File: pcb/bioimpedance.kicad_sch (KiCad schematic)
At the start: 44 parts, among them J1 Conn_01x05_Pin, J3 USB_C_Receptacle_USB2.0_16P, J6 Conn_01x16_Pin, J8 Conn_01x16_Pin, SW5 SW_Push, SW6 SW_Push, U1 ESP32-S3-WROOM-1, U2 MAX30001CWV_T, U3 AP2112K-3.3, U4 AP2112K-1.8, Y1 OK322532.768KJBA4SL

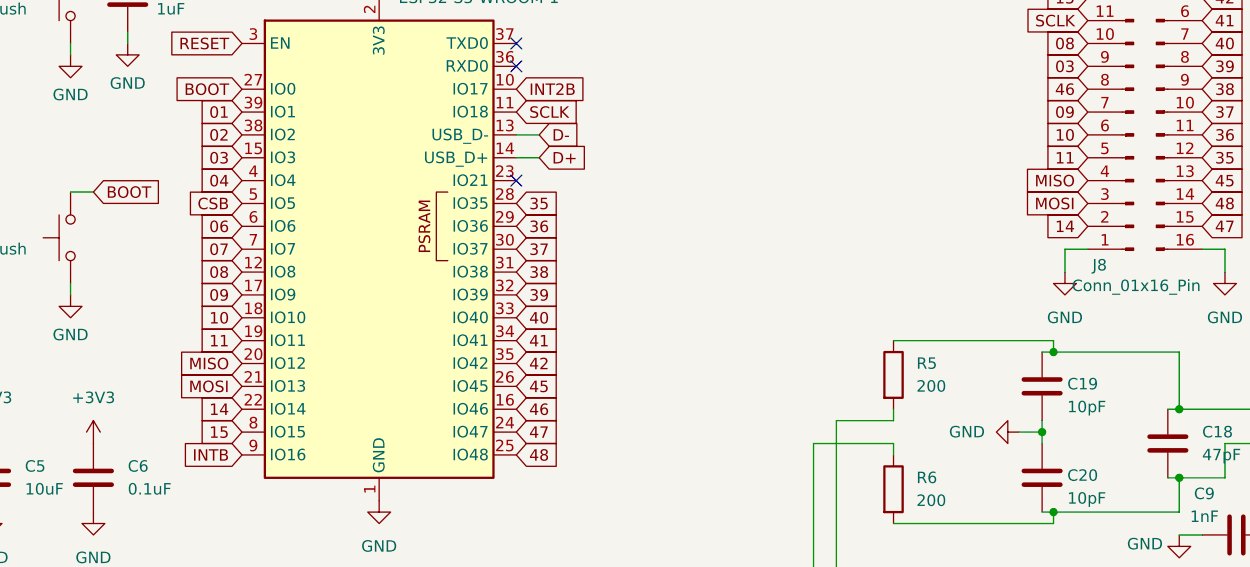
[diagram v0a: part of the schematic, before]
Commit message: reroute pcb AGAIN
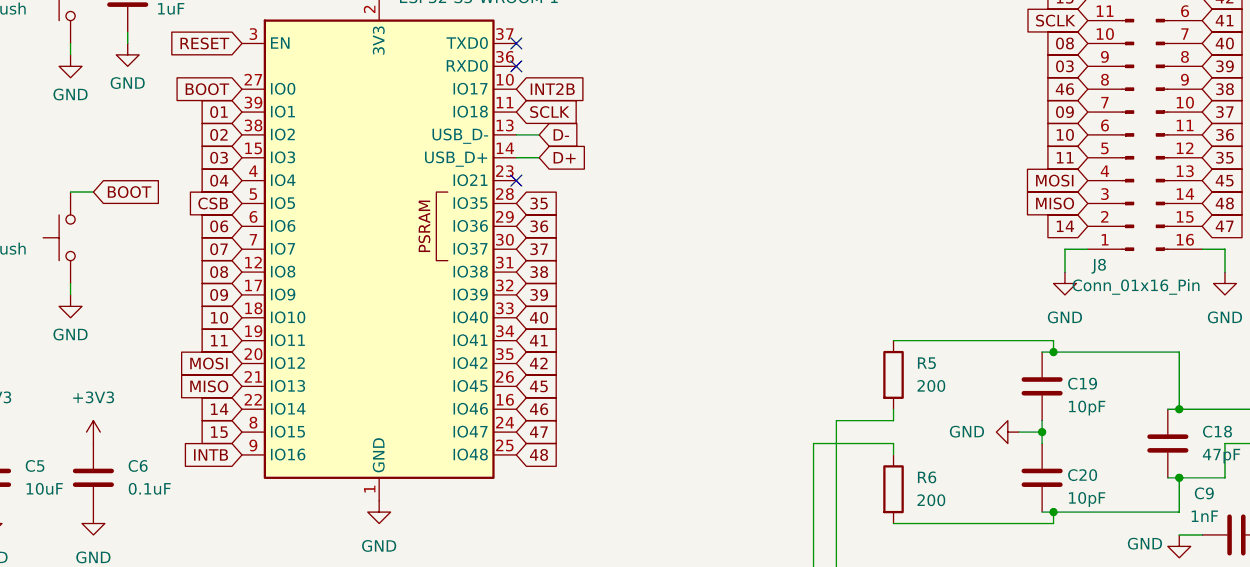
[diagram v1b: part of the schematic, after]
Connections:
- net MISO: now also J8.3 (Pin_3), U1.21 (IO13); no longer J8.4 (Pin_4), U1.20 (IO12)
- net MOSI: now also J8.4 (Pin_4), U1.20 (IO12); no longer J8.3 (Pin_3), U1.21 (IO13)

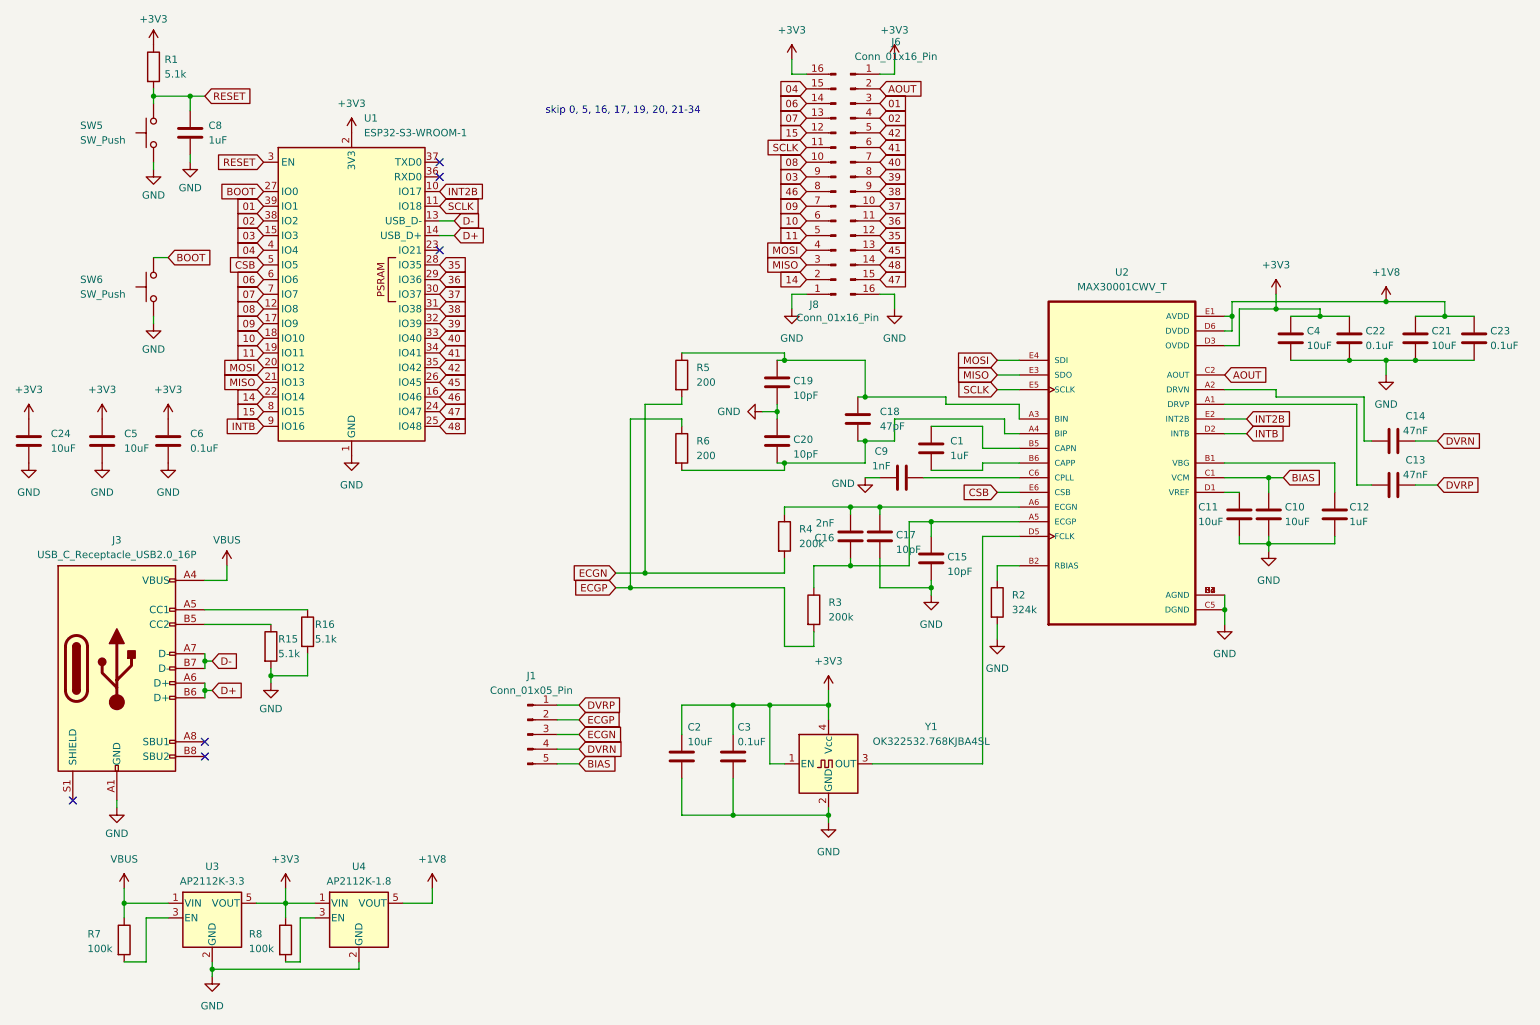
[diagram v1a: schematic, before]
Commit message: reroute board. again
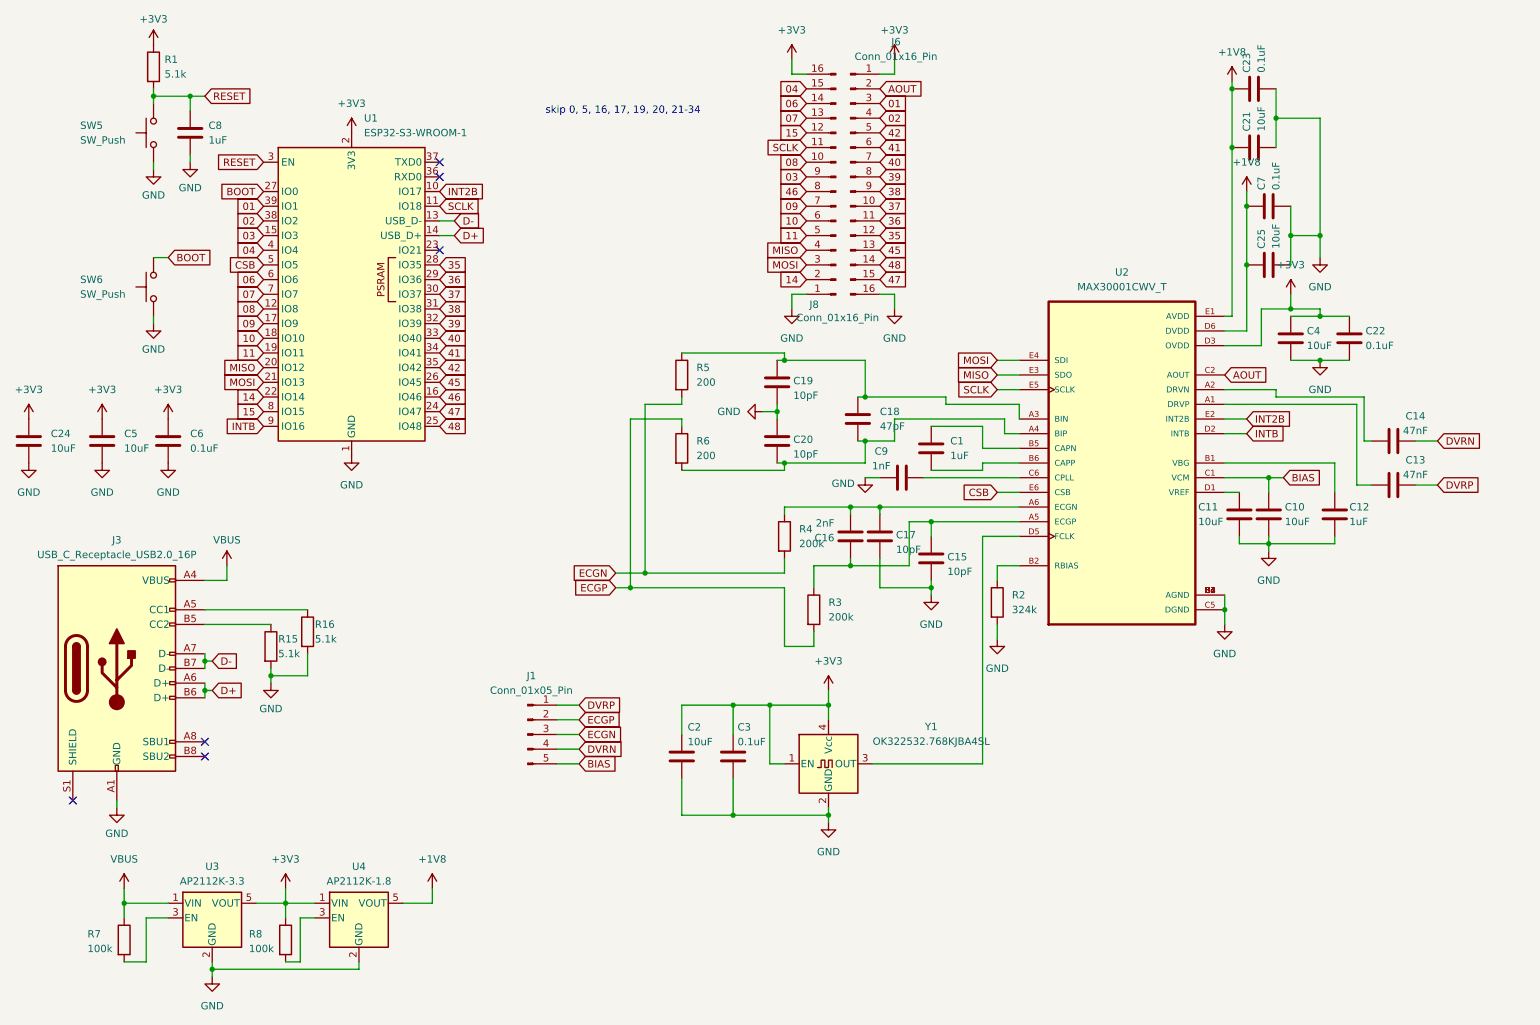
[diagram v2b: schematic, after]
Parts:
- added C25: 10uF, Capacitor_SMD:C_0805_2012Metric, symbol Device:C
- added C7: 0.1uF, Capacitor_SMD:C_0805_2012Metric, symbol Device:C
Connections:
- net +1V8: now also C25.1, C7.1
- net GND: now also C25.2, C7.2
- net MISO: now also J8.4 (Pin_4), U1.20 (IO12); no longer J8.3 (Pin_3), U1.21 (IO13)
- net MOSI: now also J8.3 (Pin_3), U1.21 (IO13); no longer J8.4 (Pin_4), U1.20 (IO12)
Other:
- moved on the sheet: C21, C23
